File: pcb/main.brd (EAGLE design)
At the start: 58.4 x 30.1 mm, 11 parts

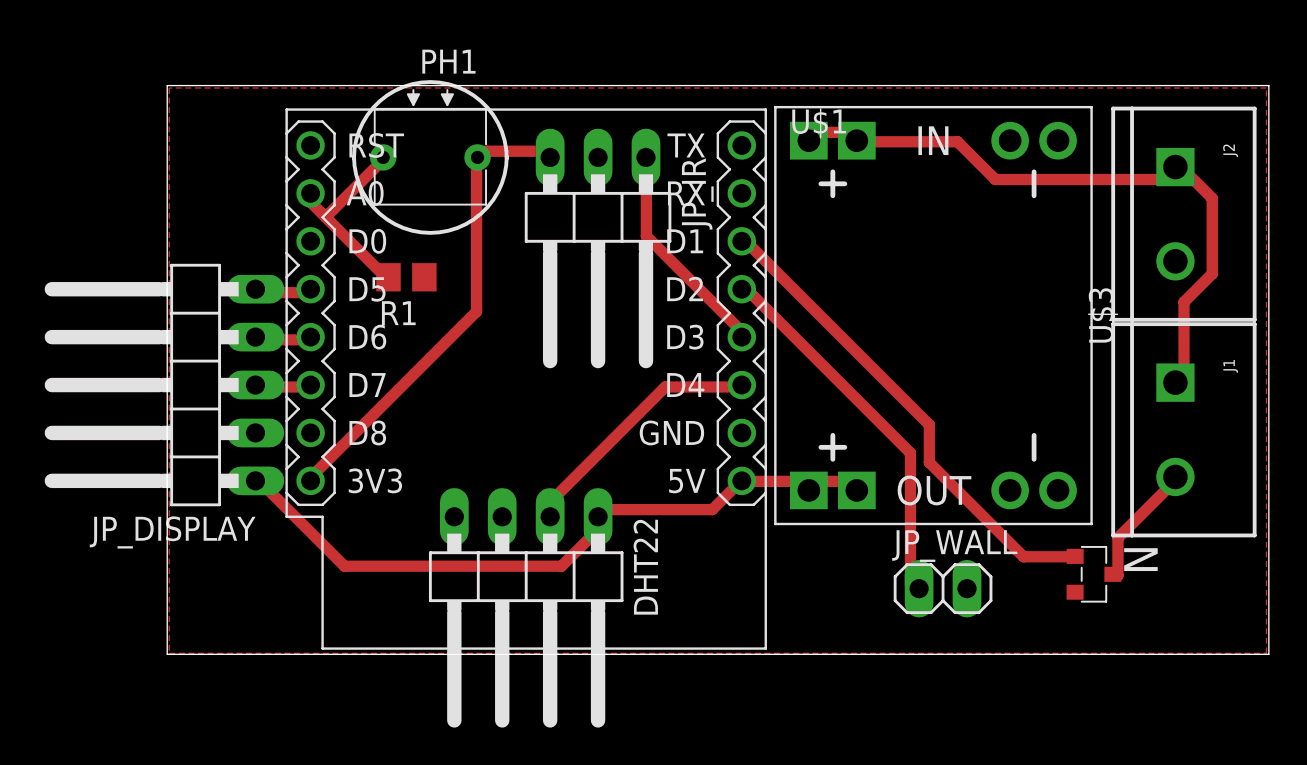
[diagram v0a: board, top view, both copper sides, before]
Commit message: upd
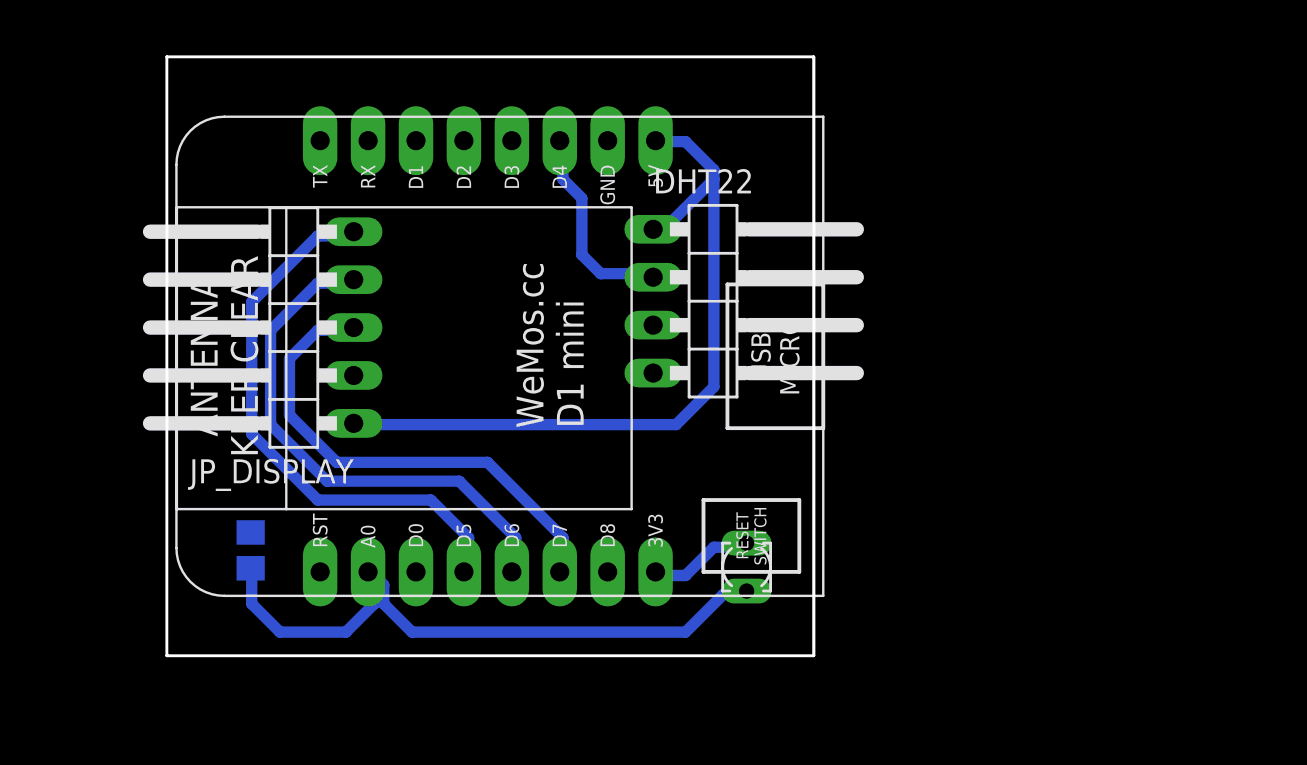
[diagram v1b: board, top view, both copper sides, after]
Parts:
- removed J1, J2: (no value), SparkFun-Connectors:SCREWTERMINAL-5MM-2
- removed JP_IR: (no value), pinhead:1X03/90
- removed JP_WALL: (no value), pinhead:1X02
- removed N: IRLML5203, transistor-power:MICRO3
- removed U$3: DC-DC-STEP-DOWN-MP1584, diy-modules:DC-DC-STEP-DOWN-MP1584
- PH1: value D1160_12 -> BPX81; device photo-elements:D11XX -> opto-trans-siemens:BPX81
- U$1: value WEMOS-D1-MINI-SHIELD -> (none); device diy-modules:WEMOS-D1-MINI-SHIELD -> esp8266modules:WEMOS-D1-MINI
- moved PH1 27.4 mm to (30.7, 4.70), turned to 90 degrees
- moved DHT22 18.5 mm to (29.6, 18.8), turned to 270 degrees
- moved R1 16.7 mm to (4.45, 5.59), flipped to the bottom, turned to 270 degrees
- moved JP_DISPLAY 6.03 mm to (6.10, 17.4)
- moved U$1 3.32 mm to (15.7, 14.6), turned to 90 degrees
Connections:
- removed net N$1: J1.1, J2.1, U$3.IN+.1, U$3.IN+.2
- removed net N$12: N.1, U$1.JP2.3
- removed net N$3: J1.2, N.3
- removed net N$5: JP_IR.1, U$1.JP2.5
- removed net N$8: JP_WALL.1, U$1.JP2.4
- net +3V3: now also PH1.C, U$1.3V3; no longer JP_IR.3, PH1.1, U$1.JP1.8
- net +5V: now also U$1.5V; no longer U$1.JP2.8, U$3.OUT+.1, U$3.OUT+.2
- net GND: now also U$1.GND; no longer J2.2, JP_IR.2, JP_WALL.2, N.2, U$1.JP2.7, U$3.IN-.1, U$3.IN-.2, U$3.OUT-.1, U$3.OUT-.2
- net N$10: now also U$1.D6; no longer U$1.JP1.5
- net N$11: now also U$1.D5; no longer U$1.JP1.4
- net N$2: now also PH1.E, U$1.A0; no longer PH1.2, U$1.JP1.2
- net N$6: now also U$1.D4; no longer U$1.JP2.6
- net N$9: now also U$1.D7; no longer U$1.JP1.6
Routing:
- net N$1: track 34.4 -> 0.00 mm
- net N$11: track 3.06 -> 29.6 mm
- net N$12: track 25.7 -> 0.00 mm
- net N$10: track 3.01 -> 27.8 mm
- net N$2: track 10.8 -> 34.0 mm
- net N$9: track 2.97 -> 26.1 mm
- net N$8: track 20.0 -> 0.00 mm
- net +3V3: track 24.8 -> 5.65 mm
- net N$5: track 11.6 -> 0.00 mm
- net N$3: track 6.76 -> 0.00 mm
- net N$6: track 13.9 -> 10.8 mm
- net +5V: track 37.3 -> 39.5 mm
- added copper zone on layer 16, net GND
- removed copper zone on layer 1, net GND
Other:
- board size 58.4 x 30.1 mm -> 34.3 x 31.8 mm
